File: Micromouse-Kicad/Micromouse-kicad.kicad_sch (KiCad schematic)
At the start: 67 parts, among them J1 UARTBTH, J2 Batería, J3 VL6180x, J4 MotorEncodL, J5 MotorEncodR, Q1 BS170, Q2 BS170, Q3 BS170, Q4 BS170, SW1 PowerSwitch, SW2 BTN, U1 YAAJ_WeAct_BlackPill_Part_Like, U2 AMS1117-5.0, U3 AMS1117-3.3, U4 MPU-6500, U5 DRV8833PWPR, U6 TCRT5000, U7 TCRT5000, U8 TCRT5000, U9 TCRT5000

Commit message: Esquemático simplificado
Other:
- note added: "Led externo y botón extra"
- note added: "Medidor - Voltaje en batería"
- note removed: "Botón Extra"
- note removed: "LEDS"
- note removed: "Voltaje Batería"
- moved on the sheet: C1, C2, C3, C4, C5, C6, C7, C8, CBOT1, CD1, CD2, CM1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

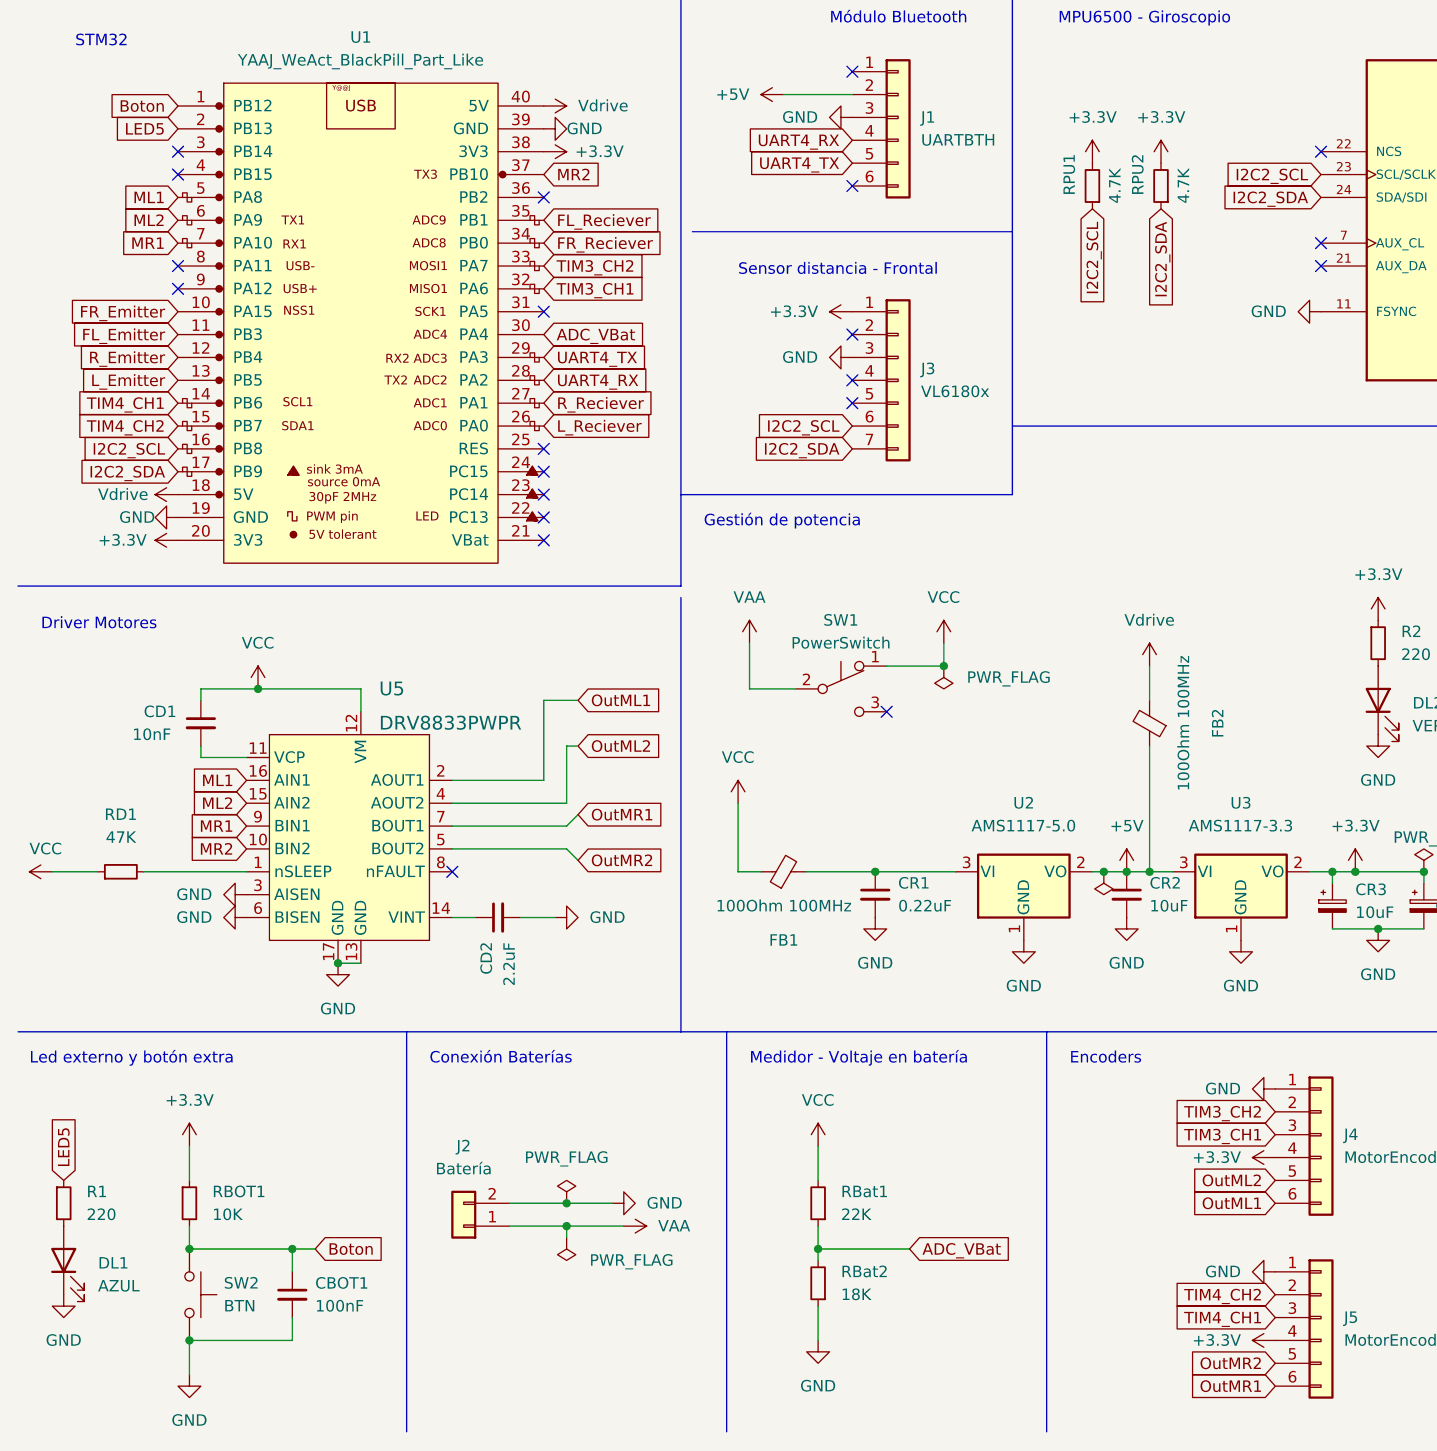
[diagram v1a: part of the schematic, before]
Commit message: Micromouse con Blackpill routeado!
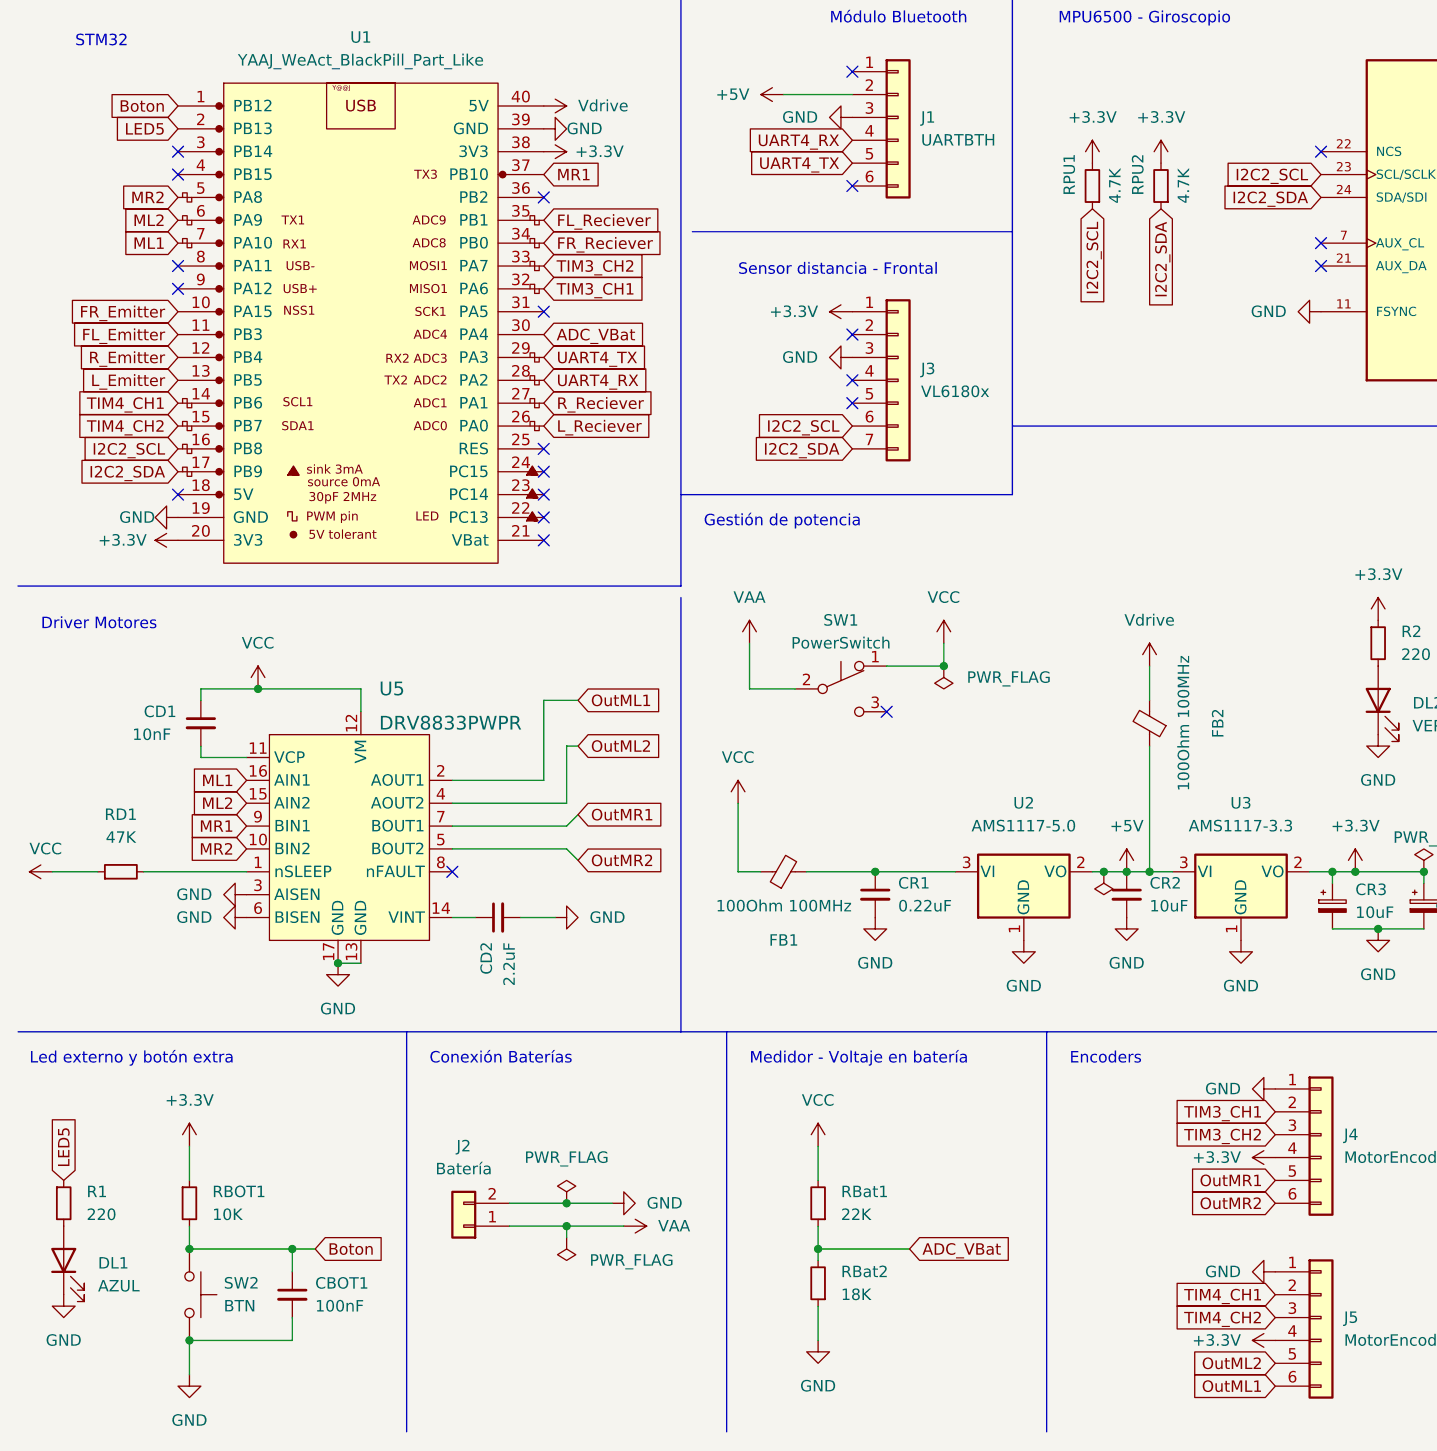
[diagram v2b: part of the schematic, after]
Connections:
- net ML1: now also U1.7 (PA10); no longer U1.5 (PA8)
- net MR1: now also U1.37 (PB10); no longer U1.7 (PA10)
- net MR2: now also U1.5 (PA8); no longer U1.37 (PB10)
- net OutML1: now also J5.6 (Pin_6); no longer J4.6 (Pin_6)
- net OutML2: now also J5.5 (Pin_5); no longer J4.5 (Pin_5)
- net OutMR1: now also J4.5 (Pin_5); no longer J5.6 (Pin_6)
- net OutMR2: now also J4.6 (Pin_6); no longer J5.5 (Pin_5)
- net TIM3_CH1: now also J4.2 (Pin_2); no longer J4.3 (Pin_3)
- net TIM3_CH2: now also J4.3 (Pin_3); no longer J4.2 (Pin_2)
- net TIM4_CH1: now also J5.2 (Pin_2); no longer J5.3 (Pin_3)
- net TIM4_CH2: now also J5.3 (Pin_3); no longer J5.2 (Pin_2)
- net Vdrive: no longer U1.18 (5V)
- no-connect marks 24 -> 25
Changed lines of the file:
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@@
   (no_connect (at 30.48 30.48))
   (no_connect (at 30.48 45.72))
+  (no_connect (at 30.48 68.58))
   (no_connect (at 30.48 43.18))
   (no_connect (at 157.48 40.64))
@@
     )
   )
-  (global_label "TIM3_CH1" (shape input) (at 152.4 139.7 180) (fields_autoplaced)
+  (global_label "TIM3_CH1" (shape input) (at 152.4 137.16 180) (fields_autoplaced)
     (effects (font (size 1.27 1.27)) (justify right))
-    (property "Intersheet References" "${INTERSHEET_REFS}" (id 0) (at 140.9759 139.6206 0)
+    (property "Intersheet References" "${INTERSHEET_REFS}" (id 0) (at 140.9759 137.0806 0)
       (effects (font (size 1.27 1.27)) (justify right) hide)
     )
@@
     )
   )
-  (global_label "OutML1" (shape input) (at 152.4 147.32 180) (fields_autoplaced)
+  (global_label "OutML1" (shape input) (at 152.4 167.64 180) (fields_autoplaced)
     (effects (font (size 1.27 1.27)) (justify right))
-    (property "Intersheet References" "${INTERSHEET_REFS}" (id 0) (at 143.0926 147.3994 0)
+    (property "Intersheet References" "${INTERSHEET_REFS}" (id 0) (at 143.0926 167.7194 0)
       (effects (font (size 1.27 1.27)) (justify right) hide)
     )
@@
     )
   )
-  (global_label "OutMR2" (shape input) (at 152.4 165.1 180) (fields_autoplaced)
+  (global_label "OutMR2" (shape input) (at 152.4 147.32 180) (fields_autoplaced)
     (effects (font (size 1.27 1.27)) (justify right))
-    (property "Intersheet References" "${INTERSHEET_REFS}" (id 0) (at 142.8507 165.0206 0)
+    (property "Intersheet References" "${INTERSHEET_REFS}" (id 0) (at 142.8507 147.2406 0)
       (effects (font (size 1.27 1.27)) (justify right) hide)
     )
@@
     )
   )
-  (global_label "OutML2" (shape input) (at 152.4 144.78 180) (fields_autoplaced)
+  (global_label "OutML2" (shape input) (at 152.4 165.1 180) (fields_autoplaced)
     (effects (font (size 1.27 1.27)) (justify right))
-    (property "Intersheet References" "${INTERSHEET_REFS}" (id 0) (at 143.0926 144.8594 0)
+    (property "Intersheet References" "${INTERSHEET_REFS}" (id 0) (at 143.0926 165.1794 0)
       (effects (font (size 1.27 1.27)) (justify right) hide)
     )
@@
     )
   )
-  (global_label "ML1" (shape input) (at 30.48 35.56 180) (fields_autoplaced)
+  (global_label "ML1" (shape input) (at 30.48 40.64 180) (fields_autoplaced)
     (effects (font (size 1.27 1.27)) (justify right))
-    (property "Intersheet References" "${INTERSHEET_REFS}" (id 0) (at 24.3779 35.6394 0)
+    (property "Intersheet References" "${INTERSHEET_REFS}" (id 0) (at 24.3779 40.7194 0)
       (effects (font (size 1.27 1.27)) (justify right) hide)
     )
@@
     )
   )
-  (global_label "TIM4_CH2" (shape input) (at 152.4 157.48 180) (fields_autoplaced)
+  (global_label "TIM4_CH2" (shape input) (at 152.4 160.02 180) (fields_autoplaced)
     (effects (font (size 1.27 1.27)) (justify right))
-    (property "Intersheet References" "${INTERSHEET_REFS}" (id 0) (at 140.9759 157.4006 0)
+    (property "Intersheet References" "${INTERSHEET_REFS}" (id 0) (at 140.9759 159.9406 0)
       (effects (font (size 1.27 1.27)) (justify right) hide)
     )
@@
     )
   )
-  (global_label "TIM4_CH1" (shape input) (at 152.4 160.02 180) (fields_autoplaced)
+  (global_label "TIM4_CH1" (shape input) (at 152.4 157.48 180) (fields_autoplaced)
     (effects (font (size 1.27 1.27)) (justify right))
-    (property "Intersheet References" "${INTERSHEET_REFS}" (id 0) (at 140.9759 159.9406 0)
+    (property "Intersheet References" "${INTERSHEET_REFS}" (id 0) (at 140.9759 157.4006 0)
       (effects (font (size 1.27 1.27)) (justify right) hide)
     )
@@
     )
   )
-  (global_label "MR1" (shape input) (at 30.48 40.64 180) (fields_autoplaced)
-    (effects (font (size 1.27 1.27)) (justify right))
-    (property "Intersheet References" "${INTERSHEET_REFS}" (id 0) (at 24.1359 40.7194 0)
-      (effects (font (size 1.27 1.27)) (justify right) hide)
+  (global_label "MR1" (shape input) (at 71.12 33.02 0) (fields_autoplaced)
+    (effects (font (size 1.27 1.27)) (justify left))
+    (property "Intersheet References" "${INTERSHEET_REFS}" (id 0) (at 77.4641 32.9406 0)
+      (effects (font (size 1.27 1.27)) (justify left) hide)
     )
   )
@@
     )
   )
-  (global_label "TIM3_CH2" (shape input) (at 152.4 137.16 180) (fields_autoplaced)
+  (global_label "TIM3_CH2" (shape input) (at 152.4 139.7 180) (fields_autoplaced)
     (effects (font (size 1.27 1.27)) (justify right))
-    (property "Intersheet References" "${INTERSHEET_REFS}" (id 0) (at 140.9759 137.0806 0)
+    (property "Intersheet References" "${INTERSHEET_REFS}" (id 0) (at 140.9759 139.6206 0)
       (effects (font (size 1.27 1.27)) (justify right) hide)
     )
   )
-  (global_label "OutMR1" (shape input) (at 152.4 167.64 180) (fields_autoplaced)
+  (global_label "OutMR1" (shape input) (at 152.4 144.78 180) (fields_autoplaced)
     (effects (font (size 1.27 1.27)) (justify right))
-    (property "Intersheet References" "${INTERSHEET_REFS}" (id 0) (at 142.8507 167.5606 0)
+    (property "Intersheet References" "${INTERSHEET_REFS}" (id 0) (at 142.8507 144.7006 0)
       (effects (font (size 1.27 1.27)) (justify right) hide)
     )
@@
     )
   )
-  (global_label "MR2" (shape input) (at 71.12 33.02 0) (fields_autoplaced)
-    (effects (font (size 1.27 1.27)) (justify left))
-    (property "Intersheet References" "${INTERSHEET_REFS}" (id 0) (at 77.4641 32.9406 0)
-      (effects (font (size 1.27 1.27)) (justify left) hide)
+  (global_label "MR2" (shape input) (at 30.48 35.56 180) (fields_autoplaced)
+    (effects (font (size 1.27 1.27)) (justify right))
+    (property "Intersheet References" "${INTERSHEET_REFS}" (id 0) (at 24.1359 35.6394 0)
+      (effects (font (size 1.27 1.27)) (justify right) hide)
     )
   )
@@
     (pin "1")
   )
-  (symbol (lib_id "power:Vdrive") (at 30.48 68.58 90) (unit 1)
-    (in_bom yes) (on_board yes)
-    (property "Reference" "#PWR02" (id 0) (at 34.29 73.66 0)
-      (effects (font (size 1.27 1.27)) hide)
-    )
-    (property "Value" "Vdrive" (id 1) (at 21.59 68.58 90)
-      (effects (font (size 1.27 1.27)) (justify right))
-    )
-    (property "Footprint" "" (id 2) (at 30.48 68.58 0)
-      (effects (font (size 1.27 1.27)) hide)
-    )
-    (property "Datasheet" "" (id 3) (at 30.48 68.58 0)
-      (effects (font (size 1.27 1.27)) hide)
-    )
-    (pin "1")
-  )
   (symbol (lib_id "Device:R_Small") (at 212.09 125.73 180) (unit 1)
     (in_bom yes) (on_board yes) (fields_autoplaced)
@@
       (reference "#PWR01") (unit 1) (value "GND") (footprint "")
     )
-    (path "/05692abd-bb2d-49f8-9485-8f3ba7662f2d"
-      (reference "#PWR02") (unit 1) (value "Vdrive") (footprint "")
-    )
     (path "/b987dcaa-12bb-4caf-b0a2-4817a69f5312"
